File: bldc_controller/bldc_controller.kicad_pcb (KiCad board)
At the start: 6 copper layers, 69.7 x 76.7 mm, 248 parts, among them J1 XT60PW-M, J10 JST S2B-PH-SM4-TB, J11 Phase A, J12 Phase B, J13 Phase C, J2 XT60PW-M, J3 SM08B-GHS-TB, J4 SM07B-GHS-TB, J5 JST S2B-PH-SM4-TB, J6 SM06B-GHS-TB, J7 Nano-Fit 1x03, J8 Nano-Fit 1x03, J9 SM05B-GHS-TB, Q1 TPH2R408QM,L1Q, Q2 TPH2R408QM,L1Q, Q3 TPH2R408QM,L1Q, Q4 TPH2R408QM,L1Q, Q5 TPH2R408QM,L1Q, Q6 TPH2R408QM,L1Q, Q7 SSM3K324R,LF, SW1 CAS-220TA, U1 SMBJ51CD-M3/H, U10 DRV8353FS, U11 SMBJ51CD-M3/H, U12 LMR36006FSCQRNXRQ1, U13 DGD0216WT-7, U2 MAX15062BATA+T, U3 ADP5301ACBZ-4-R7, U4 LP2992IM5-3.3/NOPB, U5 STM32G474RET3, U6 AS5047P, U7 AS5048B, U8 SN65HVD35DR, U9 TCAN1051HGVDRBRQ1

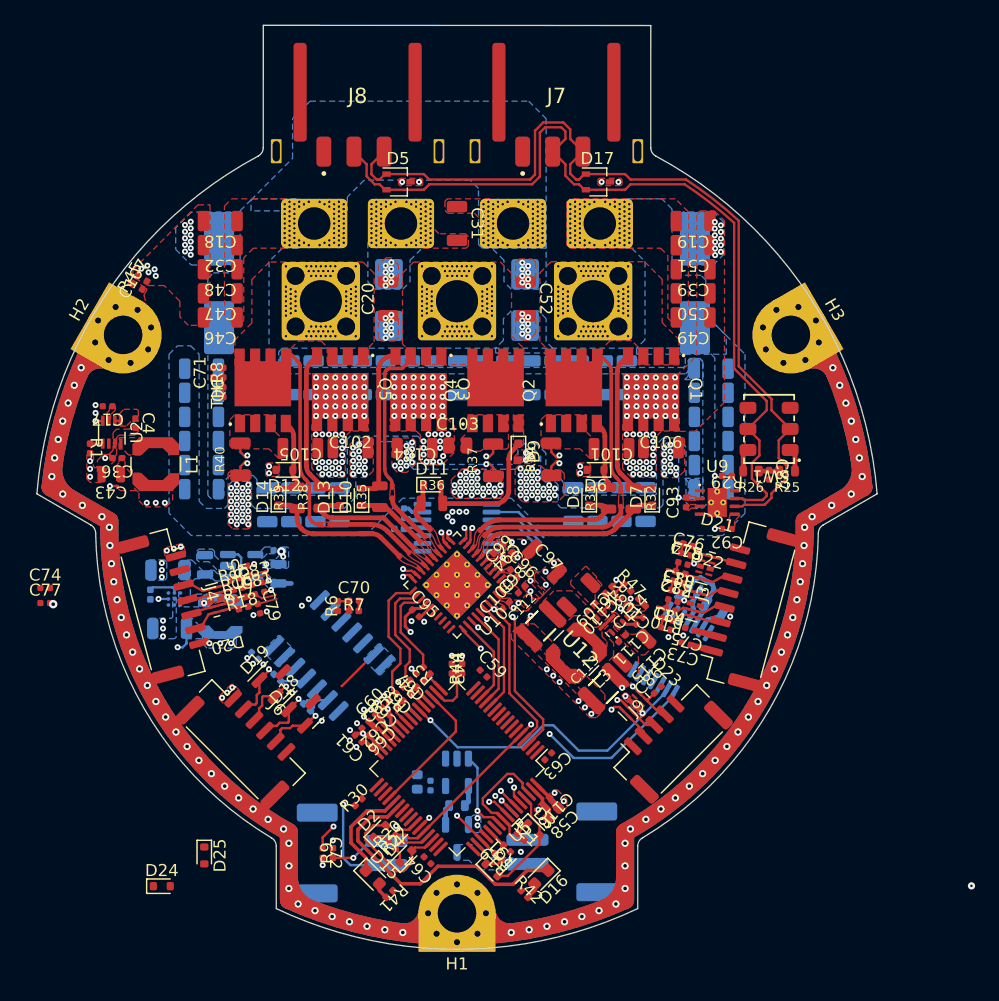
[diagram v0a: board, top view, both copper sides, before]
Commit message: might have fixed net issue, added dxf and svgs
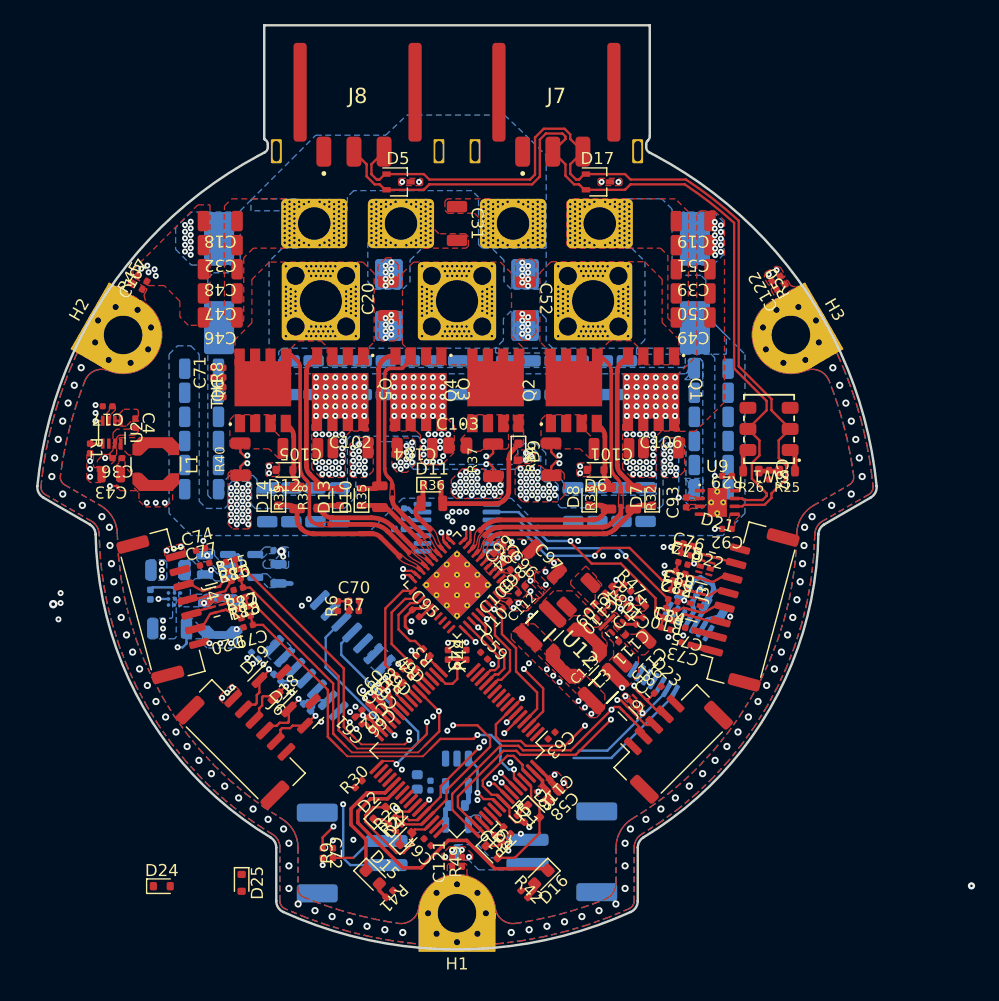
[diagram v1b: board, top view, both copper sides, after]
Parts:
- added C121: 330n, 0_capacitor_smd:C_0402_1005_DensityHigh, F.Cu at (149.5, 127.4)
- added C122: 330n, 0_capacitor_smd:C_0402_1005_DensityHigh, F.Cu at (176.2, 79.6)
- added R49: 100k, 0_resistor_smd:R_0402_1005_DensityHigh, F.Cu at (150.3, 127.4)
- added R50: 100k, 0_resistor_smd:R_0402_1005_DensityHigh, F.Cu at (176.9, 79.2)
- R23, R24: value 120R -> 100R
- moved C77 13.6 mm to (128.9, 102.7), turned to 15 degrees
- moved C74 13.3 mm to (128.6, 101.5), turned to 15 degrees
- moved D25 3.85 mm to (132.0, 129.2)
- moved C63 1.75 mm to (157.8, 117.0)
- moved C79 1.70 mm to (132.6, 107.9), turned to -165 degrees
- moved C85 1.70 mm to (131.1, 102.4), turned to -165 degrees
- moved C83 1.63 mm to (131.7, 104.8), turned to -165 degrees
- moved C81 1.63 mm to (132.0, 105.5), turned to -165 degrees
- moved C116 1.50 mm to (157.3, 120.9)
- moved C58 1.50 mm to (157.9, 121.8)
- moved C60 1.50 mm to (143.4, 113.4)
- moved C61 1.50 mm to (141.7, 115.7)
- moved C62 1.50 mm to (142.3, 114.6)
- moved C64 1.50 mm to (147.4, 125.8)
- moved C65 1.50 mm to (144.0, 114.0)
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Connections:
- net /FDCAN Transceiver/FDCAN_N renamed /Project Architecture/Interface - FD-CAN/FDCAN_N
- net /FDCAN Transceiver/FDCAN_P renamed /Project Architecture/Interface - FD-CAN/FDCAN_P
- net /FDCAN Transceiver/FDCAN_RX renamed /Project Architecture/Interface - FD-CAN/FDCAN_RX
- net /FDCAN Transceiver/FDCAN_S renamed /Project Architecture/Interface - FD-CAN/FDCAN_S
- net /FDCAN Transceiver/FDCAN_TX renamed /Project Architecture/Interface - FD-CAN/FDCAN_TX
- net /Fan Control/FAN_GATE renamed /Project Architecture/Interface - Fan Control/FAN_GATE
- net /Fan Control/FAN_OUT renamed /Project Architecture/Interface - Fan Control/FAN_OUT
- net /Fan Control/FAN_SW renamed /Project Architecture/Interface - Fan Control/FAN_SW
- net /Fan Control/FAN_~{IN} renamed /Project Architecture/Interface - Fan Control/FAN_~{IN}
- net /Interconnects/AUX1P_A renamed /Project Architecture/Interface - Interconnects/AUX1P_A
- net /Interconnects/AUX1P_B renamed /Project Architecture/Interface - Interconnects/AUX1P_B
- net /Interconnects/AUX1P_C renamed /Project Architecture/Interface - Interconnects/AUX1P_C
- net /Interconnects/AUX1P_D renamed /Project Architecture/Interface - Interconnects/AUX1P_D
- net /Interconnects/AUX1P_E renamed /Project Architecture/Interface - Interconnects/AUX1P_E
- net /Interconnects/AUX1_A renamed /Project Architecture/Interface - Interconnects/AUX1_A
- net /Interconnects/AUX1_B renamed /Project Architecture/Interface - Interconnects/AUX1_B
- net /Interconnects/AUX1_C renamed /Project Architecture/Interface - Interconnects/AUX1_C
- net /Interconnects/AUX1_D renamed /Project Architecture/Interface - Interconnects/AUX1_D
- net /Interconnects/AUX1_D_K renamed /Project Architecture/Interface - Interconnects/AUX1_D_K
- net /Interconnects/AUX1_E renamed /Project Architecture/Interface - Interconnects/AUX1_E
- net /Interconnects/AUX1_E_K renamed /Project Architecture/Interface - Interconnects/AUX1_E_K
- net /Interconnects/AUX1_I2C_PULLUP renamed /Project Architecture/Interface - Interconnects/AUX1_I2C_PULLUP
- net /Interconnects/AUX2P_A renamed /Project Architecture/Interface - Interconnects/AUX2P_A
- net /Interconnects/AUX2P_B renamed /Project Architecture/Interface - Interconnects/AUX2P_B
- net /Interconnects/AUX2P_C renamed /Project Architecture/Interface - Interconnects/AUX2P_C
- net /Interconnects/AUX2P_D renamed /Project Architecture/Interface - Interconnects/AUX2P_D
- net /Interconnects/AUX2_A renamed /Project Architecture/Interface - Interconnects/AUX2_A
- net /Interconnects/AUX2_B renamed /Project Architecture/Interface - Interconnects/AUX2_B
- net /Interconnects/AUX2_B_K renamed /Project Architecture/Interface - Interconnects/AUX2_B_K
- net /Interconnects/AUX2_C renamed /Project Architecture/Interface - Interconnects/AUX2_C
- net /Interconnects/AUX2_C_K renamed /Project Architecture/Interface - Interconnects/AUX2_C_K
- net /Interconnects/AUX2_D renamed /Project Architecture/Interface - Interconnects/AUX2_D
- net /Interconnects/AUX2_I2C_PULLUP renamed /Project Architecture/Interface - Interconnects/AUX2_I2C_PULLUP
- net /Interconnects/CAN_TERM_B renamed /Project Architecture/Interface - Interconnects/CAN_TERM_B
- net /Interconnects/CAN_TERM_MID renamed /Project Architecture/Interface - Interconnects/CAN_TERM_MID
- net /Interconnects/CAN_TERM_T renamed /Project Architecture/Interface - Interconnects/CAN_TERM_T
- net /Interconnects/NRST renamed /Project Architecture/Interface - Interconnects/NRST
- net /Interconnects/NTC_MOT_H renamed /Project Architecture/Interface - Interconnects/NTC_MOT_H
- net /Interconnects/NTC_MOT_L renamed /Project Architecture/Interface - Interconnects/NTC_MOT_L
- net /Interconnects/POS_SENSOR_CS renamed /Project Architecture/Interface - Interconnects/POS_SENSOR_CS
- net /Interconnects/RS422_D+ renamed /Project Architecture/Interface - Interconnects/RS422_D+
- net /Interconnects/RS422_D- renamed /Project Architecture/Interface - Interconnects/RS422_D-
- net /Interconnects/RS422_R+ renamed /Project Architecture/Interface - Interconnects/RS422_R+
- net /Interconnects/RS422_R- renamed /Project Architecture/Interface - Interconnects/RS422_R-
- net /Interconnects/SWCLK renamed /Project Architecture/Interface - Interconnects/SWCLK
- net /Interconnects/SWDIO renamed /Project Architecture/Interface - Interconnects/SWDIO
- net /LED Indicators/LED1 renamed /Project Architecture/MCU - IO/LED1
- net /LED Indicators/LED1_A renamed /Project Architecture/User - LED Indicators/LED1_A
- net /LED Indicators/LED2 renamed /Project Architecture/MCU - IO/LED2
- net /LED Indicators/LED2_A renamed /Project Architecture/User - LED Indicators/LED2_A
- net /Microcontroller IO/BOARD_VERSION renamed /Project Architecture/MCU - IO/BOARD_VERSION
- net /Microcontroller IO/DRV_CS renamed /Project Architecture/MCU - IO/DRV_CS
- net /Microcontroller IO/DRV_MISO renamed /Project Architecture/MCU - IO/DRV_MISO
- net /Microcontroller IO/DRV_MOSI renamed /Project Architecture/MCU - IO/DRV_MOSI
- net /Microcontroller IO/DRV_SCLK renamed /Project Architecture/MCU - IO/DRV_SCLK
- net /Microcontroller IO/FAN_CTRL renamed /Project Architecture/MCU - IO/FAN_CTRL
- net /Microcontroller IO/FILTER_SOA renamed /Project Architecture/MCU - IO/FILTER_SOA
- net /Microcontroller IO/FILTER_SOB renamed /Project Architecture/MCU - IO/FILTER_SOB
- net /Microcontroller IO/FILTER_SOC renamed /Project Architecture/MCU - IO/FILTER_SOC
- net /Microcontroller IO/MOTOR_ENABLE renamed /Project Architecture/MCU - IO/MOTOR_ENABLE
- net /Microcontroller IO/MOTOR_FAULT renamed /Project Architecture/MCU - IO/MOTOR_FAULT
- net /Microcontroller IO/MOTOR_HIZ renamed /Project Architecture/MCU - IO/MOTOR_HIZ
- net /Microcontroller IO/PWM_PHASEA renamed /Project Architecture/MCU - IO/PWM_PHASEA
- net /Microcontroller IO/PWM_PHASEB renamed /Project Architecture/MCU - IO/PWM_PHASEB
- net /Microcontroller IO/PWM_PHASEC renamed /Project Architecture/MCU - IO/PWM_PHASEC
- net /Microcontroller IO/RS422_DE renamed /Project Architecture/Interface - RS-422/RS422_DE
- net /Microcontroller IO/RS422_~{RE} renamed /Project Architecture/Interface - RS-422/RS422_~{RE}
- net /Microcontroller IO/SENSE_TEMP_FET renamed /Project Architecture/MCU - IO/SENSE_TEMP_FET
- net /Microcontroller IO/SENSE_TEMP_MOT renamed /Project Architecture/MCU - IO/SENSE_TEMP_MOT
- net /Microcontroller IO/SENSE_VBAT renamed /Project Architecture/MCU - IO/SENSE_VBAT
- net /Microcontroller IO/SOA renamed /Project Architecture/MCU - IO/SOA
- net /Microcontroller IO/SOB renamed /Project Architecture/MCU - IO/SOB
- net /Microcontroller IO/SOC renamed /Project Architecture/MCU - IO/SOC
- net /Motor Control/CPH renamed /Project Architecture/Motor Control - Top Level/CPH
- net /Motor Control/CPL renamed /Project Architecture/Motor Control - Top Level/CPL
- net /Motor Control/DVDD renamed /Project Architecture/Motor Control - Top Level/DVDD
- net /Motor Control/GHA renamed /Project Architecture/Motor Control - Top Level/GHA
- net /Motor Control/GHB renamed /Project Architecture/Motor Control - Top Level/GHB
- net /Motor Control/GHC renamed /Project Architecture/Motor Control - Top Level/GHC
- net /Motor Control/GLA renamed /Project Architecture/Motor Control - Top Level/GLA
- net /Motor Control/GLB renamed /Project Architecture/Motor Control - Top Level/GLB
- net /Motor Control/GLC renamed /Project Architecture/Motor Control - Top Level/GLC
- net /Motor Control/SA_N renamed /Project Architecture/Motor Control - Top Level/SA_N
- net /Motor Control/SA_P renamed /Project Architecture/Motor Control - Top Level/SA_P
- net /Motor Control/SB_N renamed /Project Architecture/Motor Control - Top Level/SB_N
- net /Motor Control/SB_P renamed /Project Architecture/Motor Control - Top Level/SB_P
- net /Motor Control/SC_N renamed /Project Architecture/Motor Control - Top Level/SC_N
- net /Motor Control/SC_P renamed /Project Architecture/Motor Control - Top Level/SC_P
- net /Motor Control/SHA renamed /Project Architecture/Motor Control - Top Level/SHA
- net /Motor Control/SHB renamed /Project Architecture/Motor Control - Top Level/SHB
- net /Motor Control/SHC renamed /Project Architecture/Motor Control - Top Level/SHC
- net /Motor Control/Three Phase Inverter/FET_GHA renamed /Project Architecture/Motor Control - Top Level/Motor Control - Inverter/FET_GHA
- net /Motor Control/Three Phase Inverter/FET_GHB renamed /Project Architecture/Motor Control - Top Level/Motor Control - Inverter/FET_GHB
- net /Motor Control/Three Phase Inverter/FET_GHC renamed /Project Architecture/Motor Control - Top Level/Motor Control - Inverter/FET_GHC
- net /Motor Control/Three Phase Inverter/FET_GLA renamed /Project Architecture/Motor Control - Top Level/Motor Control - Inverter/FET_GLA
- net /Motor Control/Three Phase Inverter/FET_GLB renamed /Project Architecture/Motor Control - Top Level/Motor Control - Inverter/FET_GLB
- net /Motor Control/Three Phase Inverter/FET_GLC renamed /Project Architecture/Motor Control - Top Level/Motor Control - Inverter/FET_GLC
- net /Motor Control/Three Phase Inverter/PHA renamed /Project Architecture/Motor Control - Top Level/Motor Control - Inverter/PHA
- net /Motor Control/Three Phase Inverter/PHB renamed /Project Architecture/Motor Control - Top Level/Motor Control - Inverter/PHB
- net /Motor Control/Three Phase Inverter/PHC renamed /Project Architecture/Motor Control - Top Level/Motor Control - Inverter/PHC
- net /Motor Control/Three Phase Inverter/SRC_LS_A renamed /Project Architecture/Motor Control - Top Level/Motor Control - Inverter/SRC_LS_A
- net /Motor Control/Three Phase Inverter/SRC_LS_B renamed /Project Architecture/Motor Control - Top Level/Motor Control - Inverter/SRC_LS_B
- net /Motor Control/Three Phase Inverter/SRC_LS_C renamed /Project Architecture/Motor Control - Top Level/Motor Control - Inverter/SRC_LS_C
- net /Motor Control/VCP renamed /Project Architecture/Motor Control - Top Level/VCP
- net /Motor Control/VGLS renamed /Project Architecture/Motor Control - Top Level/VGLS
- net /Position Sensors/COMM_VDD renamed /Project Architecture/Sensing - Position/COMM_VDD
- net /Position Sensors/DIS_VDD3V renamed /Project Architecture/Sensing - Position/DIS_VDD3V
- net /Power Generation/ADJ_A3V3 renamed /Project Architecture/Power - Generation/ADJ_A3V3
- net /Power Generation/BOOT_12V renamed /Project Architecture/Power - Generation/BOOT_12V
- net /Power Generation/FB_12V renamed /Project Architecture/Power - Generation/FB_12V
- net /Power Generation/FB_3V3 renamed /Project Architecture/Power - Generation/FB_3V3
- net /Power Generation/FB_5V renamed /Project Architecture/Power - Generation/FB_5V
- net /Power Generation/FB_DIV_12V renamed /Project Architecture/Power - Generation/FB_DIV_12V
- net /Power Generation/LX_5V renamed /Project Architecture/Power - Generation/LX_5V
- net /Power Generation/MODE_3V3 renamed /Project Architecture/Power - Generation/MODE_3V3
- net /Power Generation/MODE_5V renamed /Project Architecture/Power - Generation/MODE_5V
- net /Power Generation/PG_12V renamed /Project Architecture/Power - Generation/PG_12V
- net /Power Generation/PG_3V3 renamed /Project Architecture/Power - Generation/PG_3V3
- net /Power Generation/SW_12V renamed /Project Architecture/Power - Generation/SW_12V
- net /Power Generation/SW_3V3 renamed /Project Architecture/Power - Generation/SW_3V3
- net /Power Generation/VCC_12V renamed /Project Architecture/Power - Generation/VCC_12V
- net /Power Generation/VCC_5V renamed /Project Architecture/Power - Generation/VCC_5V
- net /Power Generation/VID_3V3 renamed /Project Architecture/Power - Generation/VID_3V3
- net /Power Generation/~{RST}_5V renamed /Project Architecture/Power - Generation/~{RST}_5V
- J4 pad MP: (no net) -> CHASSIS
- J9 pad MP: (no net) -> CHASSIS
- U5 pad 10: unconnected-(U5B-PC2-Pad10) -> /Project Architecture/MCU - IO/PC1
- U5 pad 11: unconnected-(U5B-PC3-Pad11) -> /Project Architecture/MCU - IO/PC3
- U5 pad 23: unconnected-(U5B-PC5-Pad23) -> /Project Architecture/MCU - IO/PC5
- U5 pad 39: unconnected-(U5B-PC7-Pad39) -> /Project Architecture/MCU - IO/PC7
- U5 pad 40: unconnected-(U5B-PC8-Pad40) -> /Project Architecture/MCU - IO/PC8
- U5 pad 41: unconnected-(U5B-PC9-Pad41) -> /Project Architecture/MCU - IO/PC9
- U5 pad 54: unconnected-(U5B-PC12-Pad54) -> /Project Architecture/MCU - IO/PC12
- U5 pad 8: unconnected-(U5B-PC0-Pad8) -> /Project Architecture/MCU - IO/PC0
- U5 pad 9: unconnected-(U5B-PC1-Pad9) -> /Project Architecture/MCU - IO/PC1
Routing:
- net CHASSIS: track 991.3 -> 0.00 mm
- net /Project Architecture/Interface - Interconnects/AUX2_A: track 2.28 -> 35.8 mm, vias 0 -> 2
- net /Project Architecture/Interface - Interconnects/AUX2_D: track 3.91 -> 33.4 mm, vias 1 -> 2
- net /Project Architecture/Interface - Interconnects/AUX1_E: track 12.7 -> 41.9 mm, vias 0 -> 2
- net /Project Architecture/Interface - Interconnects/AUX2_C: track 30.8 -> 54.8 mm, vias 1 -> 2
- net /Project Architecture/Interface - Interconnects/AUX2_B: track 33.3 -> 56.4 mm, vias 2 -> 3
- net /Project Architecture/Interface - Interconnects/SWCLK: track 3.92 -> 24.6 mm, vias 1 -> 2
- net /Project Architecture/Interface - Interconnects/SWDIO: track 3.94 -> 24.2 mm
- net /Project Architecture/Interface - Interconnects/NRST: track 4.19 -> 23.1 mm, vias 1 -> 3
- net /Project Architecture/Interface - RS-422/RS422_DE: track 0.00 -> 16.6 mm, vias 0 -> 1
- net /Project Architecture/Interface - RS-422/RS422_~{RE}: track 0.00 -> 13.5 mm, vias 0 -> 1
- net /Project Architecture/Interface - Interconnects/AUX1_C: track 5.40 -> 18.3 mm, vias 0 -> 1
- net GND: track 16.6 -> 29.0 mm, vias 234 -> 252
- net /Project Architecture/Interface - Interconnects/AUX1_B: track 8.38 -> 20.2 mm, vias 1 -> 2
- net /Project Architecture/MCU - IO/MOTOR_ENABLE: track 18.0 -> 12.3 mm
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- added copper zone on B.Cu, net CHASSIS
- added copper zone on In1.Cu, net CHASSIS
- added copper zone on In2.Cu, net CHASSIS
- added copper zone on In3.Cu, net CHASSIS
- added copper zone on In4.Cu, net CHASSIS
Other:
- outline, holes or cut-outs redrawn
